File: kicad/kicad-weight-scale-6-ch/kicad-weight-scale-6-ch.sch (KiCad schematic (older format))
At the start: 44 parts, among them J1 Barrel_Jack_Switch, J2 Conn_01x02, J3 Conn_01x04, J4 Conn_01x04, J5 Conn_01x04, J6 Conn_01x02, J7 Conn_01x02, J8 Conn_01x02, J9 Conn_01x02, Q1 Si4542DY, Q2 Si4542DY, Q3 AO3401A, SW1 SW_Push, U1 TP-4056, U10 USB_Type_C, U11 USB_Type_C, U12 USB_Type_C, U13 USB_Type_C, U2 StepUpTo5V, U3 WCMCU-ADS1232, U4 ESPWROOM32, U5 WCMCU-ADS1232, U6 DataLoggingBoard, U7 WCMCU-ADS1232, U8 USB_Type_C, U9 USB_Type_C

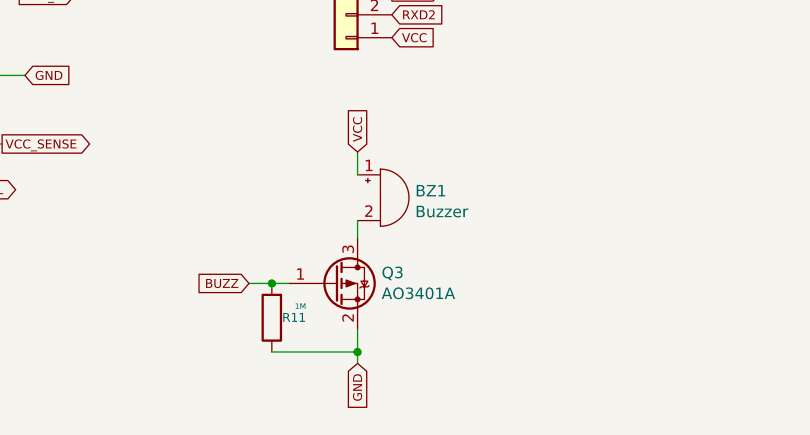
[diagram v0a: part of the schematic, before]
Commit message: Update nextion-esp32dws6chwl_ench.HMI, kicad-weight-scale-6-ch-cache.lib, and 6 more files...
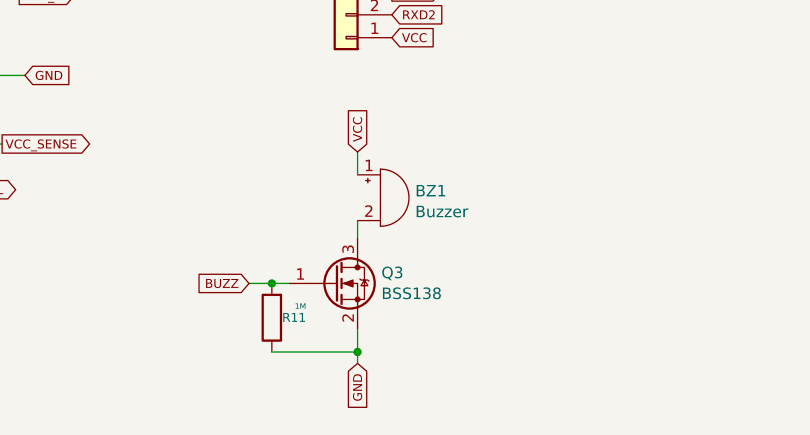
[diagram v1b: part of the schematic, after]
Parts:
- removed Q3: AO3401A, Package_TO_SOT_SMD:SOT-23, symbol Transistor_FET:AO3401A
- added Q3: BSS138, Package_TO_SOT_SMD:SOT-23, symbol Transistor_FET:BSS138
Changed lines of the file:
@@
-$EndComp
-$Comp
-L Transistor_FET:AO3401A Q3
-U 1 1 606F53CC
-P 3800 6700
-F 0 "Q3" H 4005 6746 50  0000 L CNN
-F 1 "AO3401A" H 4005 6655 50  0000 L CNN
-F 2 "Package_TO_SOT_SMD:SOT-23" H 4000 6625 50  0001 L CIN
-F 3 "http://www.aosmd.com/pdfs/datasheet/AO3401A.pdf" H 3800 6700 50  0001 L CNN
-	1    3800 6700
-	1    0    0    -1
 $EndComp
 $Comp
@@
 	2540 1650 2750 1650
 Connection ~ 2540 2030
+$Comp
+L Transistor_FET:BSS138 Q3
+U 1 1 60917343
+P 3800 6700
+F 0 "Q3" H 4004 6746 50  0000 L CNN
+F 1 "BSS138" H 4004 6655 50  0000 L CNN
+F 2 "Package_TO_SOT_SMD:SOT-23" H 4000 6625 50  0001 L CIN
+F 3 "https://www.onsemi.com/pub/Collateral/BSS138-D.PDF" H 3800 6700 50  0001 L CNN
+	1    3800 6700
+	1    0    0    -1
+$EndComp
 $EndSCHEMATC
